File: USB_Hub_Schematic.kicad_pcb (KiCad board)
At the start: 4 copper layers, 0 parts

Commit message: PCB Layout
Initial layout finished, subject to routing
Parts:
- added C1: 0.1 uF, Capacitor_SMD:C_0603_1608Metric, F.Cu at (150.0, 110.2)
- added C12: 47 uF, Capacitor_SMD:C_0805_2012Metric, F.Cu at (148.8, 76.0)
- added C13: 47 uF, Capacitor_SMD:C_0805_2012Metric, F.Cu at (146.8, 76.0)
- added C14: 12 pF, Capacitor_SMD:C_0603_1608Metric, F.Cu at (140.8, 80.5)
- added C15: 10 uF, Capacitor_SMD:C_0805_2012Metric, F.Cu at (140.1, 66.3)
- added C17: 47 uF, Capacitor_SMD:C_0805_2012Metric, F.Cu at (146.8, 66.7)
- added C18: 0.1 uF, Capacitor_SMD:C_0603_1608Metric, F.Cu at (161.6, 75.8)
- added C19: 33 uF, Capacitor_SMD:C_0805_2012Metric, F.Cu at (162.6, 82.6)
- added C2: 12 pF, Capacitor_SMD:C_0603_1608Metric, F.Cu at (148.5, 103.3)
- added C20: 1 uF, Capacitor_SMD:C_0805_2012Metric, F.Cu at (143.6, 99.7)
- added C21: 12 pF, Capacitor_SMD:C_0603_1608Metric, F.Cu at (135.2, 83.5)
- added C22: 1 uF, Capacitor_SMD:C_0805_2012Metric, F.Cu at (138.0, 85.5)
- added C23: 0.1 uF, Capacitor_SMD:C_0603_1608Metric, F.Cu at (135.9, 91.0)
- added C24: 0.1 uF, Capacitor_SMD:C_0603_1608Metric, F.Cu at (134.7, 86.0)
- added C25: 0.1 uF, Capacitor_SMD:C_0603_1608Metric, F.Cu at (146.7, 85.8)
- added C26: 1 uF, Capacitor_SMD:C_0805_2012Metric, F.Cu at (145.0, 103.5)
- added C27: 1 uF, Capacitor_SMD:C_0805_2012Metric, F.Cu at (139.1, 112.5)
- added C28: 4.7 uF, Capacitor_SMD:C_0805_2012Metric, F.Cu at (151.2, 93.5)
- added C29: 0.1 uF, Capacitor_SMD:C_0603_1608Metric, F.Cu at (141.4, 85.7)
- added C3: 12 pF, Capacitor_SMD:C_0603_1608Metric, F.Cu at (147.0, 103.3)
- added C30: 33 uF, Capacitor_SMD:C_0805_2012Metric, F.Cu at (159.4, 110.5)
- added C31: 1 uF, Capacitor_SMD:C_0805_2012Metric, F.Cu at (135.5, 88.5)
- added C32: 0.1 uF, Capacitor_SMD:C_0603_1608Metric, F.Cu at (149.4, 87.5)
- added C33: 47 uF, Capacitor_SMD:C_0805_2012Metric, F.Cu at (150.8, 76.0)
- added C34: 33 uF, Capacitor_SMD:C_0805_2012Metric, F.Cu at (162.5, 73.0)
- added C35: 1 uF, Capacitor_SMD:C_0805_2012Metric, F.Cu at (140.7, 99.0)
- added C36: 0.1 uF, Capacitor_SMD:C_0603_1608Metric, F.Cu at (140.9, 100.8)
- added C37: 0.1 uF, Capacitor_SMD:C_0603_1608Metric, F.Cu at (152.8, 76.2)
- added C38: 47 uF, Capacitor_SMD:C_0805_2012Metric, F.Cu at (148.8, 66.7)
- added C39: 47 uF, Capacitor_SMD:C_0805_2012Metric, F.Cu at (150.8, 66.7)
- added C4: 1 uF, Capacitor_SMD:C_0805_2012Metric, F.Cu at (136.9, 72.9)
- added C40: 0.1 uF, Capacitor_SMD:C_0603_1608Metric, F.Cu at (152.8, 66.9)
- added C41: 0.1 uF, Capacitor_SMD:C_0603_1608Metric, F.Cu at (137.0, 117.8)
- added C42: 0.1 uF, Capacitor_SMD:C_0603_1608Metric, F.Cu at (147.5, 117.8)
- added C43: 100 uF, Capacitor_SMD:C_1206_3216Metric, F.Cu at (149.5, 117.0)
- added C44: 0.1 uF, Capacitor_SMD:C_0603_1608Metric, F.Cu at (147.5, 121.4)
- added C45: 100 uF, Capacitor_SMD:C_1206_3216Metric, F.Cu at (149.5, 122.2)
- added C46: 1 uF, Capacitor_SMD:C_0805_2012Metric, F.Cu at (139.0, 103.5)
- added C47: 1 uF, Capacitor_SMD:C_0805_2012Metric, F.Cu at (141.0, 103.5)
- added C48: 33 uF, Capacitor_SMD:C_0805_2012Metric, F.Cu at (159.4, 121.8)
- added C49: 0.1 uF, Capacitor_SMD:C_0603_1608Metric, F.Cu at (161.6, 66.0)
- added C5: 4.7 uF, Capacitor_SMD:C_0805_2012Metric, F.Cu at (140.1, 72.3)
- added C6: 10 uF, Capacitor_SMD:C_0805_2012Metric, F.Cu at (140.1, 70.3)
- added C7: 10 uF, Capacitor_SMD:C_0805_2012Metric, F.Cu at (140.1, 68.3)
- added C8: 100 pF, Capacitor_SMD:C_0603_1608Metric, F.Cu at (143.6, 66.3)
- added C9: 0.1 uF, Capacitor_SMD:C_0603_1608Metric, F.Cu at (136.0, 93.0)
- added Card1: microSD Reader, lcsc_easyeda:TF-SMD_TF-PUSH, F.Cu at (165.5, 92.5)
- added D1: LED, LED_SMD:LED_0805_2012Metric, F.Cu at (139.1, 106.5)
- added D10: LED, LED_SMD:LED_0805_2012Metric, F.Cu at (154.9, 81.0)
- added D11: LED, LED_SMD:LED_0805_2012Metric, F.Cu at (150.8, 79.0)
- added D12: LED, LED_SMD:LED_0805_2012Metric, F.Cu at (150.8, 69.6)
- added D13: LED, LED_SMD:LED_0805_2012Metric, F.Cu at (154.8, 71.6)
- added D14: LED, LED_SMD:LED_0805_2012Metric, F.Cu at (152.0, 121.6)
- added D15: LED, LED_SMD:LED_0805_2012Metric, F.Cu at (152.0, 117.6)
- added D16: LED, LED_SMD:LED_0805_2012Metric, F.Cu at (140.1, 115.6)
- added D17: LED, LED_SMD:LED_0805_2012Metric, F.Cu at (140.0, 123.6)
- added J1: USB-C, Connector_Wire:SolderWire-0.1sqmm_1x04_P3.6mm_D0.4mm_OD1mm_Relief, F.Cu at (116.9, 119.5)
- added J2: USB-A, Connector_Wire:SolderWire-0.1sqmm_1x04_P3.6mm_D0.4mm_OD1mm_Relief, F.Cu at (127.5, 71.5)
- added L1: 0.47 uH, Inductor_SMD:L_1008_2520Metric, F.Cu at (143.5, 70.9)
- added R1: 100k, Resistor_SMD:R_0603_1608Metric, F.Cu at (158.7, 78.0)
- added R10: 33k, Resistor_SMD:R_0603_1608Metric, F.Cu at (133.3, 77.6)
- added R11: 10k, Resistor_SMD:R_0603_1608Metric, F.Cu at (135.8, 77.6)
- added R12: 40k, Resistor_SMD:R_0603_1608Metric, F.Cu at (131.0, 77.3)
- added R13: 10k, Resistor_SMD:R_0603_1608Metric, F.Cu at (131.0, 75.8)
- added R14: 40k, Resistor_SMD:R_0603_1608Metric, F.Cu at (132.5, 72.8)
- added R15: 10k, Resistor_SMD:R_0603_1608Metric, F.Cu at (131.0, 74.3)
- added R16: 100k, Resistor_SMD:R_0603_1608Metric, F.Cu at (137.3, 77.6)
- added R17: 12k, Resistor_SMD:R_0603_1608Metric, F.Cu at (140.7, 83.5)
- added R18: 453k, Resistor_SMD:R_0603_1608Metric, F.Cu at (143.6, 67.8)
- added R19: 100k, Resistor_SMD:R_0603_1608Metric, F.Cu at (144.1, 74.5)
- added R2: 100k, Resistor_SMD:R_0603_1608Metric, F.Cu at (159.0, 68.6)
- added R20: 100k, Resistor_SMD:R_0603_1608Metric, F.Cu at (141.5, 76.3)
- added R21: 1k, Resistor_SMD:R_0603_1608Metric, F.Cu at (151.5, 114.3)
- added R23: 1k, Resistor_SMD:R_0603_1608Metric, F.Cu at (158.3, 81.0)
- added R24: 10k, Resistor_SMD:R_0603_1608Metric, F.Cu at (144.3, 82.0)
- added R25: 10k, Resistor_SMD:R_0603_1608Metric, F.Cu at (144.3, 85.0)
- added R26: 10k, Resistor_SMD:R_0603_1608Metric, F.Cu at (144.3, 83.5)
- added R27: 10k, Resistor_SMD:R_0603_1608Metric, F.Cu at (148.5, 89.8)
- added R28: 10k, Resistor_SMD:R_0603_1608Metric, F.Cu at (150.0, 97.3)
- added R29: 10k, Resistor_SMD:R_0603_1608Metric, F.Cu at (136.7, 95.8)
- added R3: 10k, Resistor_SMD:R_0603_1608Metric, F.Cu at (146.0, 116.4)
- added R30: 1k, Resistor_SMD:R_0603_1608Metric, F.Cu at (143.3, 123.6)
- added R31: 1k, Resistor_SMD:R_0603_1608Metric, F.Cu at (143.3, 115.6)
- added R32: 330, Resistor_SMD:R_0603_1608Metric, F.Cu at (163.1, 75.8)
- added R33: 330, Resistor_SMD:R_0603_1608Metric, F.Cu at (163.1, 66.0)
- added R34: 100k, Resistor_SMD:R_0603_1608Metric, F.Cu at (150.0, 89.8)
- added R37: 10k, Resistor_SMD:R_0603_1608Metric, F.Cu at (151.5, 89.8)
- added R38: 10k, Resistor_SMD:R_0603_1608Metric, F.Cu at (148.2, 97.3)
- added R4: 10k, Resistor_SMD:R_0603_1608Metric, F.Cu at (146.0, 122.9)
- added R41: 10k, Resistor_SMD:R_0603_1608Metric, F.Cu at (151.5, 97.3)
- added R46: 10k, Resistor_SMD:R_0603_1608Metric, F.Cu at (144.3, 86.5)
- added R47: 100k, Resistor_SMD:R_0603_1608Metric, F.Cu at (149.3, 93.3)
- added R48: 1M, Resistor_SMD:R_1206_3216Metric, F.Cu at (138.0, 82.0)
- added R49: 100k, Resistor_SMD:R_0603_1608Metric, F.Cu at (158.7, 79.5)
- added R51: 100k, Resistor_SMD:R_0603_1608Metric, F.Cu at (151.0, 81.0)
- added R52: 1k, Resistor_SMD:R_0603_1608Metric, F.Cu at (147.3, 79.0)
- added R53: 1k, Resistor_SMD:R_0603_1608Metric, F.Cu at (147.3, 69.6)
- added R54: 100k, Resistor_SMD:R_0603_1608Metric, F.Cu at (151.0, 71.6)
- added R55: 1k, Resistor_SMD:R_0603_1608Metric, F.Cu at (158.3, 71.6)
- added R56: 100k, Resistor_SMD:R_0603_1608Metric, F.Cu at (159.0, 70.1)
- added R57: 1k, Resistor_SMD:R_0603_1608Metric, F.Cu at (151.5, 124.9)
- added R6: 10k, Resistor_SMD:R_0603_1608Metric, F.Cu at (138.1, 109.3)
- added R7: 12k, Resistor_SMD:R_0603_1608Metric, F.Cu at (143.0, 103.7)
- added R8: 10k, Resistor_SMD:R_0603_1608Metric, F.Cu at (149.2, 112.5)
- added R9: 40k, Resistor_SMD:R_0603_1608Metric, F.Cu at (138.2, 75.3)
- added U1: USB2517 Chip, lcsc_easyeda:QFN-64_L9.0-W9.0-P0.50-BL-EP4.8, F.Cu at (142.5, 92.5)
- added U10: TP, lcsc_easyeda:TEST-SMD_L2.7-W1.0, F.Cu at (136.5, 67.5)
- added U11: TP, lcsc_easyeda:TEST-SMD_L2.7-W1.0, F.Cu at (134.5, 99.5)
- added U12: TP, lcsc_easyeda:TEST-SMD_L2.7-W1.0, F.Cu at (134.5, 103.0)
- added U13: TP, lcsc_easyeda:TEST-SMD_L2.7-W1.0, F.Cu at (155.0, 86.0)
- added U14: TP, lcsc_easyeda:TEST-SMD_L2.7-W1.0, F.Cu at (155.0, 91.8)
- added U15: TP, lcsc_easyeda:TEST-SMD_L2.7-W1.0, F.Cu at (155.0, 98.0)
- added U16: TPS25821, lcsc_easyeda:WSON-12_L3.0-W2.0-P0.5-BL-EP, F.Cu at (155.3, 78.2)
- added U17: TPS25821, lcsc_easyeda:WSON-12_L3.0-W2.0-P0.5-BL-EP, F.Cu at (155.4, 69.0)
- added U2: USB to microSD, lcsc_easyeda:QFN-36_L6.0-W6.0-P0.50-EP4.2, F.Cu at (144.5, 109.5)
- added U3: MUX, lcsc_easyeda:VQFN-HR-12_L2.5-W2.0-P0.50-BL, F.Cu at (134.3, 74.8)
- added U5: 3.3V CONV, lcsc_easyeda:VSON-6_L1.5-W1.5-P0.50-TL, F.Cu at (142.4, 74.3)
- added U7: TPS2052B, lcsc_easyeda:SOIC-8_L4.9-W3.9-P1.27-LS6.0-BL, F.Cu at (141.5, 119.6)
- added U9: TP, lcsc_easyeda:TEST-SMD_L2.7-W1.0, F.Cu at (132.5, 70.0)
- added USB5: USB-C F, lcsc_easyeda:TYPE-C-TH_TYPE-C-14P-CC-2.6, F.Cu at (165.1, 79.5)
- added USB6: USB-A F, lcsc_easyeda:USB-A-TH_USB-226-BRY, F.Cu at (159.6, 106.0)
- added USB7: USB-A F, lcsc_easyeda:USB-A-TH_USB-226-BRY, F.Cu at (159.6, 117.2)
- added USB8: USB-C F, lcsc_easyeda:TYPE-C-TH_TYPE-C-14P-CC-2.6, F.Cu at (165.1, 69.6)
- added X1: 24MHz, lcsc_easyeda:CRYSTAL-SMD_4P-L2.0-W1.6-BL-A, F.Cu at (149.5, 106.5)
- added X2: 24MHz, lcsc_easyeda:CRYSTAL-SMD_4P-L2.0-W1.6-BL-A, F.Cu at (135.5, 81.1)
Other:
- board outline added: 60.5 x 63 mm

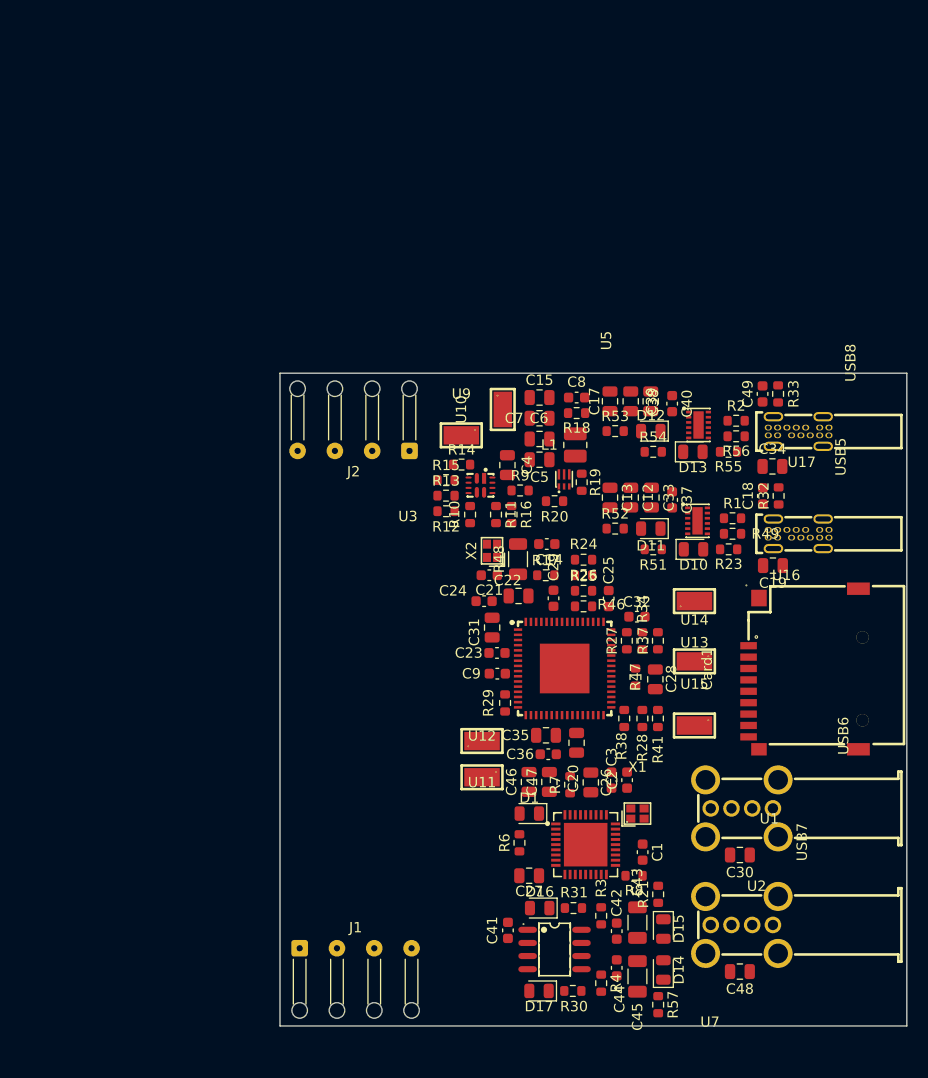
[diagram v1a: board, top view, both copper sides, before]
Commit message: Routing
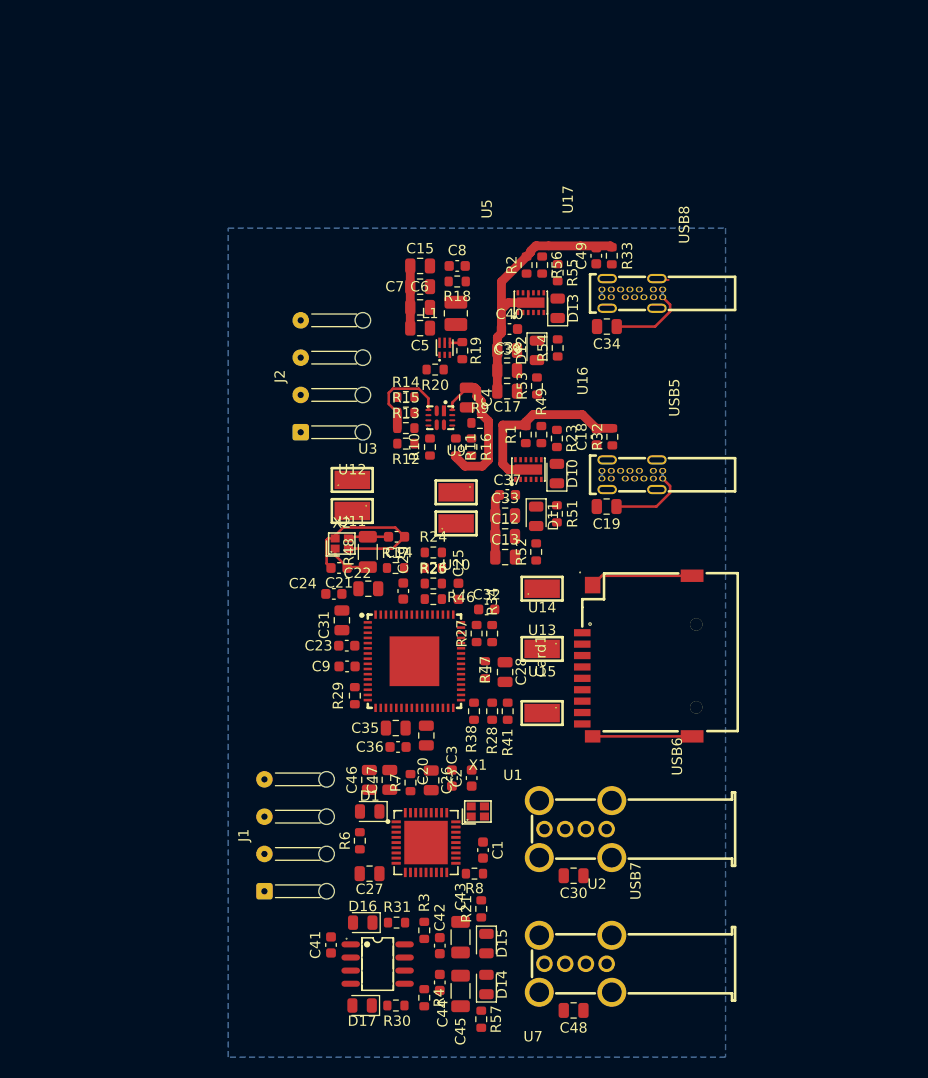
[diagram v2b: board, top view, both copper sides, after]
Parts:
- removed R37: 10k, Resistor_SMD:R_0603_1608Metric
- moved U12 28.6 mm to (122.0, 77.3)
- moved U11 28.1 mm to (122.0, 74.3)
- moved R2 25.2 mm to (138.8, 53.6), turned to 90 degrees
- moved R56 25.0 mm to (140.3, 53.6), turned to -90 degrees
- moved R55 23.9 mm to (141.8, 54.3), turned to -90 degrees
- moved R1 21.5 mm to (138.7, 69.9), turned to 90 degrees
- moved C34 20.9 mm to (146.6, 59.5), turned to 180 degrees
- moved USB8 20.9 mm to (149.0, 56.3)
- moved C49 20.9 mm to (145.5, 52.7)
- moved R33 20.9 mm to (147.0, 52.7)
- moved R49 20.8 mm to (140.2, 69.9), turned to -90 degrees
- moved U17 20.0 mm to (139.2, 57.2), turned to 0 degrees
- moved R23 19.7 mm to (141.7, 70.3), turned to -90 degrees
- moved D13 19.0 mm to (141.8, 57.7), turned to 90 degrees
- moved C40 17.3 mm to (137.2, 59.7), turned to 0 degrees
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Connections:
- U1 pad 45: /TP_SUSPIND -> /3.3V_GLOBAL
- U13 pad 1: /TP_SUSPIND -> /3.3V_GLOBAL
- U17 pad 3: GND -> /5V_OUT
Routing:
- net GND: track 0.00 -> 137.8 mm
- net /IC_X_OUT: track 0.00 -> 4.35 mm
- net /1M: track 0.00 -> 4.26 mm
- net Net-(C49-Pad1): track 0.00 -> 2.02 mm
- added copper zone on B.Cu, net GND
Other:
- board outline removed
- copper layers 4 -> 2

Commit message: Routing
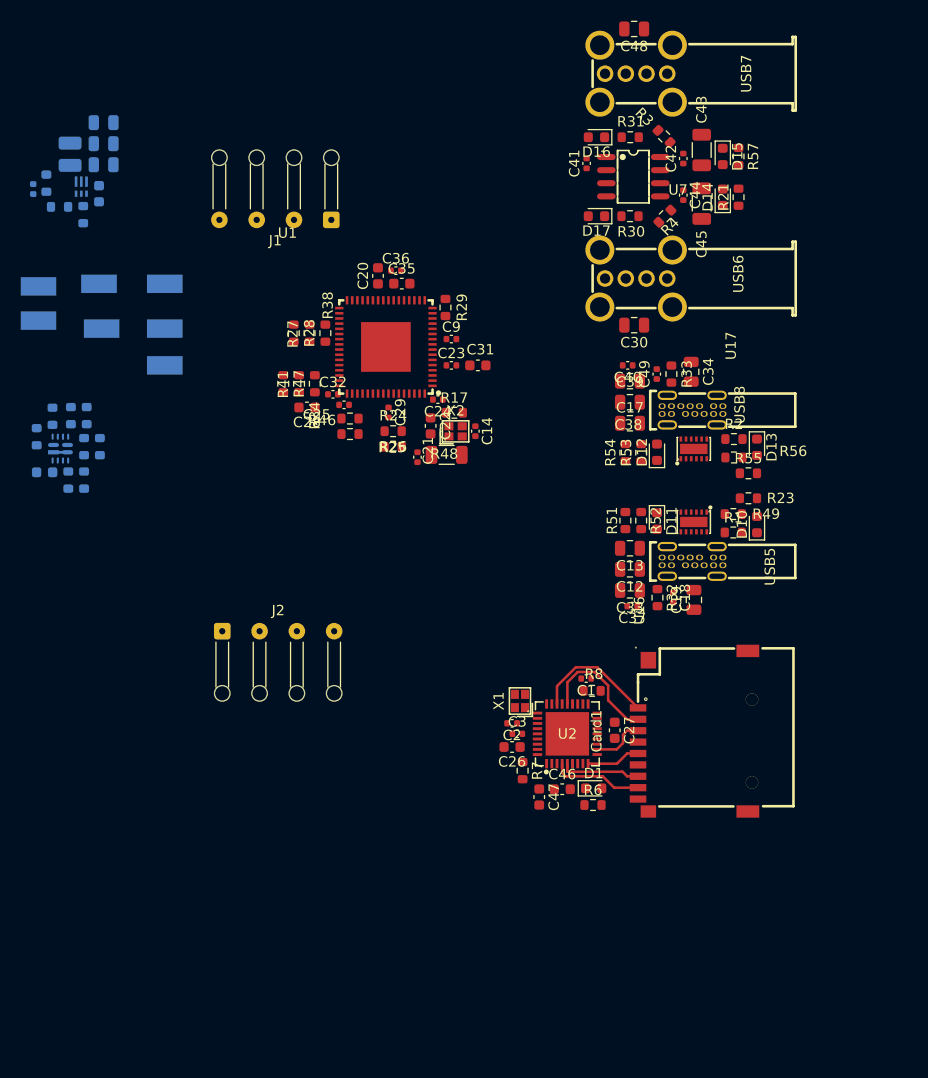
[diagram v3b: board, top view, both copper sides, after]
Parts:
- C1, C14, C18, C2, C21, C23, C24, C25, C29, C3, C32, C36, C37, C40, C41, C42, C44, C49, C9: footprint Capacitor_SMD:C_0603_1608Metric -> Capacitor_SMD:C_0402_1005Metric
- C15, C6, C7, L1, R10, R11, R12, R13, R14, R15, R16, R18, R19, R20, R9, U10, U11, U12, U13, U14, U15, U3, U5, U9: moved to B.Cu
- C20, C22, C26, C27, C28, C31, C35, C46, C47: footprint Capacitor_SMD:C_0805_2012Metric -> Capacitor_SMD:C_0603_1608Metric
- C4, C5: footprint Capacitor_SMD:C_0805_2012Metric -> Capacitor_SMD:C_0603_1608Metric; moved to B.Cu
- C8: footprint Capacitor_SMD:C_0603_1608Metric -> Capacitor_SMD:C_0402_1005Metric; moved to B.Cu
- D1, D10, D11, D12, D13, D14, D15, D16, D17: footprint LED_SMD:LED_0805_2012Metric -> LED_SMD:LED_0603_1608Metric
- moved C48 94.9 mm to (149.2, 30.8)
- moved R57 86.9 mm to (159.3, 43.1)
- moved USB7 86.1 mm to (149.4, 35.1)
- moved R3 80.0 mm to (152.1, 41.2), turned to 135 degrees
- moved U7 79.9 mm to (149.1, 45.0)
- moved C44 79.5 mm to (153.9, 46.8)
- moved C42 79.5 mm to (153.9, 43.3)
- moved C45 79.5 mm to (155.7, 47.6)
- moved D17 79.5 mm to (145.5, 48.8)
- moved R30 79.5 mm to (148.8, 48.8)
- moved C43 79.5 mm to (155.7, 42.5)
- moved C41 79.4 mm to (144.6, 43.8)
- moved D14 79.3 mm to (157.7, 47.0)
- moved D15 79.3 mm to (157.7, 43.1)
- moved R31 79.1 mm to (148.8, 41.2)
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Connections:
- C42 pad 1: /PORT4 -> /PORT5
- C43 pad 1: /PORT4 -> /PORT5
- C44 pad 1: /PORT5 -> /PORT4
- C45 pad 1: /PORT5 -> /PORT4
- D14 pad 2: /PORT5 -> /PORT4
- D15 pad 2: /PORT4 -> /PORT5
- R3 pad 1: /OC4 -> /OC5
- R30 pad 2: /OC5 -> /OC4
- R31 pad 2: /OC4 -> /OC5
- R4 pad 1: /OC5 -> /OC4
- U7 pad 3: /PWR4 -> /PWR5
- U7 pad 4: /PWR5 -> /PWR4
- U7 pad 5: /OC5 -> /OC4
- U7 pad 6: /PORT5 -> /PORT4
- U7 pad 7: /PORT4 -> /PORT5
- U7 pad 8: /OC4 -> /OC5
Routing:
- net GND: track 137.8 -> 0.61 mm
- net /SD_D3: track 0.00 -> 12.1 mm
- net /SD_D2: track 0.00 -> 11.9 mm
- net /SD_D1: track 0.00 -> 8.79 mm
- net /SD_D0: track 0.00 -> 7.76 mm
- net /SD_CLK: track 0.00 -> 5.23 mm
- net /SD_CMD: track 0.00 -> 5.16 mm
- net /IC_X_OUT: track 4.35 -> 0.00 mm
- net /1M: track 4.26 -> 0.00 mm
- net Net-(C49-Pad1): track 2.02 -> 0.00 mm
- net /5V_OUT: track 0.00 -> 1.35 mm
- removed copper zone on B.Cu, net GND
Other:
- copper layers 2 -> 4
